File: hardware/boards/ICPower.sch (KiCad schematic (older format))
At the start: 47 parts, among them U1 ECP5UM5G-381caBGA, U3 CYUSB3014, U4 IS43TR16256B-125KBL, U5 128MiB, U6 128MiB, U7 SI5330B

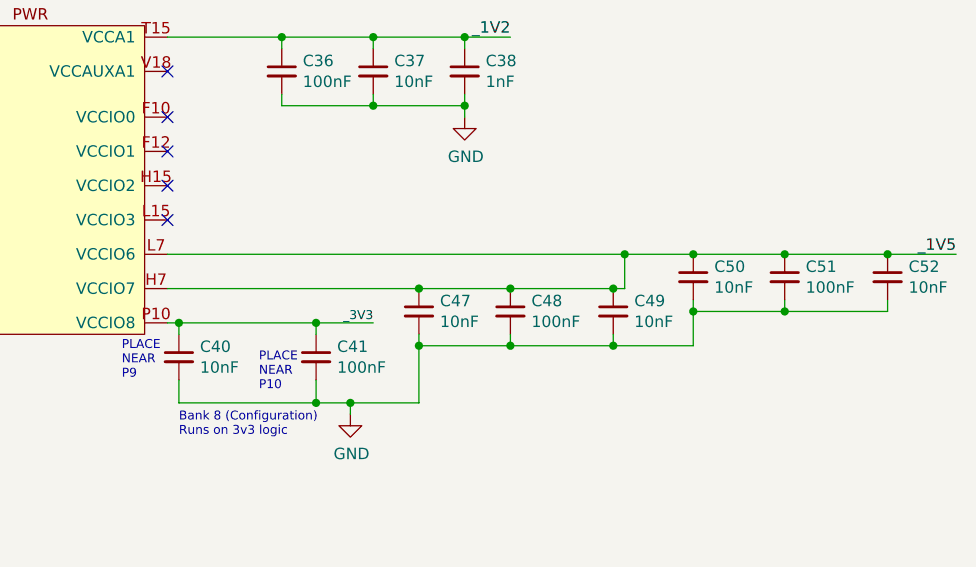
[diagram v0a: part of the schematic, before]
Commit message: A batch of misc changes, I don't exactly recall what changed
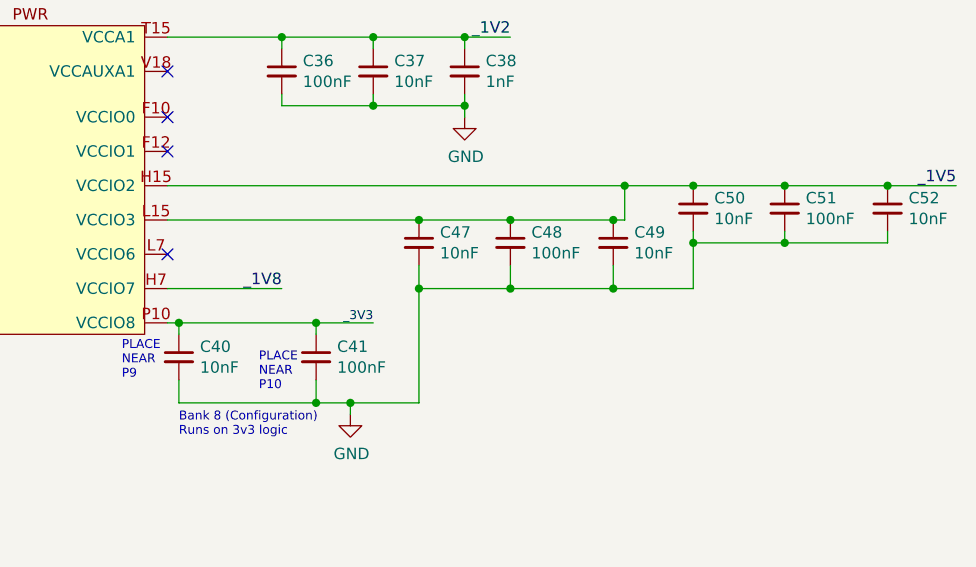
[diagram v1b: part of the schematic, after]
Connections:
- net 1V5: now also U1.H14 (VCCIO2), U1.H15 (VCCIO2), U1.J15 (VCCIO2), U1.L14 (VCCIO3), U1.L15 (VCCIO3), U1.M15 (VCCIO3); no longer U1.H6 (VCCIO7), U1.H7 (VCCIO7), U1.J6 (VCCIO7), U1.L6 (VCCIO6), U1.L7 (VCCIO6), U1.M6 (VCCIO6)
- net 1V8: now also U1.H6 (VCCIO7), U1.H7 (VCCIO7), U1.J6 (VCCIO7)
- new net: U1.L6 (VCCIO6), U1.L7 (VCCIO6), U1.M6 (VCCIO6)
- no-connect marks 9 -> 8
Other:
- moved on the sheet: C47, C48, C49, C50, C51, C52
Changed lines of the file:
@@
 NoConn ~ 9100 2000
 NoConn ~ 9100 2150
-NoConn ~ 9100 2300
-NoConn ~ 9100 2450
 $Comp
 L Device:C_Small C40
@@
 	9700 8000 9750 8000
 Wire Wire Line
-	9100 2750 10200 2750
-Wire Wire Line
-	9100 2600 11100 2600
-Wire Wire Line
-	11100 2750 11100 2600
-Connection ~ 11100 2600
-Wire Wire Line
-	11100 2600 11400 2600
-Text Label 12550 2600 2    50   ~ 0
+	9100 2450 10200 2450
+Wire Wire Line
+	9100 2300 11100 2300
+Wire Wire Line
+	11100 2450 11100 2300
+Connection ~ 11100 2300
+Wire Wire Line
+	11100 2300 11400 2300
+Text Label 12550 2300 2    50   ~ 0
 _1V5
 $Comp
 L Device:C_Small C48
 U 1 1 5FA901F7
-P 10600 2850
-F 0 "C48" H 10692 2896 50  0000 L CNN
-F 1 "100nF" H 10692 2805 50  0000 L CNN
-F 2 "Capacitor_SMD:C_0402_1005Metric" H 10600 2850 50  0001 C CNN
-F 3 "~" H 10600 2850 50  0001 C CNN
-F 4 "KEMET" H 10600 2850 50  0001 C CNN "MFR"
-F 5 "C0402C104M8PACTU" H 10600 2850 50  0001 C CNN "MPN"
-	1    10600 2850
-	1    0    0    -1
-$EndComp
-Connection ~ 10600 2750
-Wire Wire Line
-	10600 2750 11050 2750
+P 10600 2550
+F 0 "C48" H 10692 2596 50  0000 L CNN
+F 1 "100nF" H 10692 2505 50  0000 L CNN
+F 2 "Capacitor_SMD:C_0402_1005Metric" H 10600 2550 50  0001 C CNN
+F 3 "~" H 10600 2550 50  0001 C CNN
+F 4 "KEMET" H 10600 2550 50  0001 C CNN "MFR"
+F 5 "C0402C104M8PACTU" H 10600 2550 50  0001 C CNN "MPN"
+	1    10600 2550
+	1    0    0    -1
+$EndComp
+Connection ~ 10600 2450
+Wire Wire Line
+	10600 2450 11050 2450
 $Comp
 L Device:C_Small C47
 U 1 1 5FA94FC6
-P 10200 2850
-F 0 "C47" H 10292 2896 50  0000 L CNN
-F 1 "10nF" H 10292 2805 50  0000 L CNN
-F 2 "Capacitor_SMD:C_0402_1005Metric" H 10200 2850 50  0001 C CNN
-F 3 "~" H 10200 2850 50  0001 C CNN
-F 4 "KEMET" H 10200 2850 50  0001 C CNN "MFR"
-F 5 "C0402C103M5RACTU" H 10200 2850 50  0001 C CNN "MPN"
-	1    10200 2850
-	1    0    0    -1
-$EndComp
-Connection ~ 10200 2750
-Wire Wire Line
-	10200 2750 10600 2750
+P 10200 2550
+F 0 "C47" H 10292 2596 50  0000 L CNN
+F 1 "10nF" H 10292 2505 50  0000 L CNN
+F 2 "Capacitor_SMD:C_0402_1005Metric" H 10200 2550 50  0001 C CNN
+F 3 "~" H 10200 2550 50  0001 C CNN
+F 4 "KEMET" H 10200 2550 50  0001 C CNN "MFR"
+F 5 "C0402C103M5RACTU" H 10200 2550 50  0001 C CNN "MPN"
+	1    10200 2550
+	1    0    0    -1
+$EndComp
+Connection ~ 10200 2450
+Wire Wire Line
+	10200 2450 10600 2450
 $Comp
 L Device:C_Small C49
 U 1 1 5FABEDAF
-P 11050 2850
-F 0 "C49" H 11142 2896 50  0000 L CNN
-F 1 "10nF" H 11142 2805 50  0000 L CNN
-F 2 "Capacitor_SMD:C_0402_1005Metric" H 11050 2850 50  0001 C CNN
-F 3 "~" H 11050 2850 50  0001 C CNN
-F 4 "KEMET" H 11050 2850 50  0001 C CNN "MFR"
-F 5 "C0402C103M5RACTU" H 11050 2850 50  0001 C CNN "MPN"
-	1    11050 2850
-	1    0    0    -1
-$EndComp
-Connection ~ 11050 2750
-Wire Wire Line
-	11050 2750 11100 2750
-Wire Wire Line
-	10200 2950 10200 3000
-Wire Wire Line
-	10200 3000 10600 3000
-Wire Wire Line
-	11050 3000 11050 2950
-Wire Wire Line
-	10600 2950 10600 3000
-Connection ~ 10600 3000
-Wire Wire Line
-	10600 3000 11050 3000
-Wire Wire Line
-	10200 3000 10200 3250
+P 11050 2550
+F 0 "C49" H 11142 2596 50  0000 L CNN
+F 1 "10nF" H 11142 2505 50  0000 L CNN
+F 2 "Capacitor_SMD:C_0402_1005Metric" H 11050 2550 50  0001 C CNN
+F 3 "~" H 11050 2550 50  0001 C CNN
+F 4 "KEMET" H 11050 2550 50  0001 C CNN "MFR"
+F 5 "C0402C103M5RACTU" H 11050 2550 50  0001 C CNN "MPN"
+	1    11050 2550
+	1    0    0    -1
+$EndComp
+Connection ~ 11050 2450
+Wire Wire Line
+	11050 2450 11100 2450
+Wire Wire Line
+	10200 2750 10600 2750
+Wire Wire Line
+	11050 2750 11050 2650
+Wire Wire Line
+	10600 2650 10600 2750
+Connection ~ 10600 2750
+Wire Wire Line
+	10600 2750 11050 2750
 Wire Wire Line
 	10200 3250 9900 3250
-Connection ~ 10200 3000
 Connection ~ 9900 3250
 $Comp
 L Device:C_Small C51
 U 1 1 5FAD68A7
-P 11800 2700
-F 0 "C51" H 11892 2746 50  0000 L CNN
-F 1 "100nF" H 11892 2655 50  0000 L CNN
-F 2 "Capacitor_SMD:C_0402_1005Metric" H 11800 2700 50  0001 C CNN
-F 3 "~" H 11800 2700 50  0001 C CNN
-F 4 "KEMET" H 11800 2700 50  0001 C CNN "MFR"
-F 5 "C0402C104M8PACTU" H 11800 2700 50  0001 C CNN "MPN"
-	1    11800 2700
+P 11800 2400
+F 0 "C51" H 11892 2446 50  0000 L CNN
+F 1 "100nF" H 11892 2355 50  0000 L CNN
+F 2 "Capacitor_SMD:C_0402_1005Metric" H 11800 2400 50  0001 C CNN
+F 3 "~" H 11800 2400 50  0001 C CNN
+F 4 "KEMET" H 11800 2400 50  0001 C CNN "MFR"
+F 5 "C0402C104M8PACTU" H 11800 2400 50  0001 C CNN "MPN"
+	1    11800 2400
 	1    0    0    -1
 $EndComp
@@
 L Device:C_Small C50
 U 1 1 5FAD68AF
-P 11400 2700
-F 0 "C50" H 11492 2746 50  0000 L CNN
-F 1 "10nF" H 11492 2655 50  0000 L CNN
-F 2 "Capacitor_SMD:C_0402_1005Metric" H 11400 2700 50  0001 C CNN
-F 3 "~" H 11400 2700 50  0001 C CNN
-F 4 "KEMET" H 11400 2700 50  0001 C CNN "MFR"
-F 5 "C0402C103M5RACTU" H 11400 2700 50  0001 C CNN "MPN"
-	1    11400 2700
+P 11400 2400
+F 0 "C50" H 11492 2446 50  0000 L CNN
+F 1 "10nF" H 11492 2355 50  0000 L CNN
+F 2 "Capacitor_SMD:C_0402_1005Metric" H 11400 2400 50  0001 C CNN
+F 3 "~" H 11400 2400 50  0001 C CNN
+F 4 "KEMET" H 11400 2400 50  0001 C CNN "MFR"
+F 5 "C0402C103M5RACTU" H 11400 2400 50  0001 C CNN "MPN"
+	1    11400 2400
 	1    0    0    -1
 $EndComp
@@
 L Device:C_Small C52
 U 1 1 5FAD68B7
-P 12250 2700
-F 0 "C52" H 12342 2746 50  0000 L CNN
-F 1 "10nF" H 12342 2655 50  0000 L CNN
-F 2 "Capacitor_SMD:C_0402_1005Metric" H 12250 2700 50  0001 C CNN
-F 3 "~" H 12250 2700 50  0001 C CNN
-F 4 "KEMET" H 12250 2700 50  0001 C CNN "MFR"
-F 5 "C0402C103M5RACTU" H 12250 2700 50  0001 C CNN "MPN"
-	1    12250 2700
-	1    0    0    -1
-$EndComp
-Connection ~ 11400 2600
-Wire Wire Line
-	11400 2600 11800 2600
-Connection ~ 11800 2600
-Wire Wire Line
-	11800 2600 12250 2600
-Connection ~ 12250 2600
-Wire Wire Line
-	12250 2600 12550 2600
-Wire Wire Line
-	11400 2800 11400 2850
-Wire Wire Line
-	11400 2850 11800 2850
-Wire Wire Line
-	12250 2850 12250 2800
-Wire Wire Line
-	11800 2800 11800 2850
-Connection ~ 11800 2850
-Wire Wire Line
-	11800 2850 12250 2850
-Wire Wire Line
-	11050 3000 11400 3000
-Wire Wire Line
-	11400 3000 11400 2850
-Connection ~ 11050 3000
-Connection ~ 11400 2850
+P 12250 2400
+F 0 "C52" H 12342 2446 50  0000 L CNN
+F 1 "10nF" H 12342 2355 50  0000 L CNN
+F 2 "Capacitor_SMD:C_0402_1005Metric" H 12250 2400 50  0001 C CNN
+F 3 "~" H 12250 2400 50  0001 C CNN
+F 4 "KEMET" H 12250 2400 50  0001 C CNN "MFR"
+F 5 "C0402C103M5RACTU" H 12250 2400 50  0001 C CNN "MPN"
+	1    12250 2400
+	1    0    0    -1
+$EndComp
+Connection ~ 11400 2300
+Wire Wire Line
+	11400 2300 11800 2300
+Connection ~ 11800 2300
+Wire Wire Line
+	11800 2300 12250 2300
+Connection ~ 12250 2300
+Wire Wire Line
+	12250 2300 12550 2300
+Wire Wire Line
+	11400 2500 11400 2550
+Wire Wire Line
+	11400 2550 11800 2550
+Wire Wire Line
+	12250 2550 12250 2500
+Wire Wire Line
+	11800 2500 11800 2550
+Connection ~ 11800 2550
+Wire Wire Line
+	11800 2550 12250 2550
+Wire Wire Line
+	11050 2750 11400 2750
+Wire Wire Line
+	11400 2750 11400 2550
+Connection ~ 11050 2750
+Connection ~ 11400 2550
 $Comp
 L Device:C_Small C?
@@
 Wire Wire Line
 	5950 8700 6350 8700
+Wire Wire Line
+	10200 2750 10200 3250
+Wire Wire Line
+	10200 2650 10200 2750
+Connection ~ 10200 2750
+Text Label 9600 2750 2    50   ~ 0
+_1V8
+Wire Wire Line
+	9100 2750 9600 2750
+NoConn ~ 9100 2600
 $EndSCHEMATC
